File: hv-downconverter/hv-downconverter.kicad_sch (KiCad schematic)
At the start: 24 parts, among them J1 Conn_01x02_Pin, J2 Conn_01x02_Pin, Q3 Q_NMOS_GSD, Q4 Q_NMOS_GSD, U1 LM5116MHX/NOPB

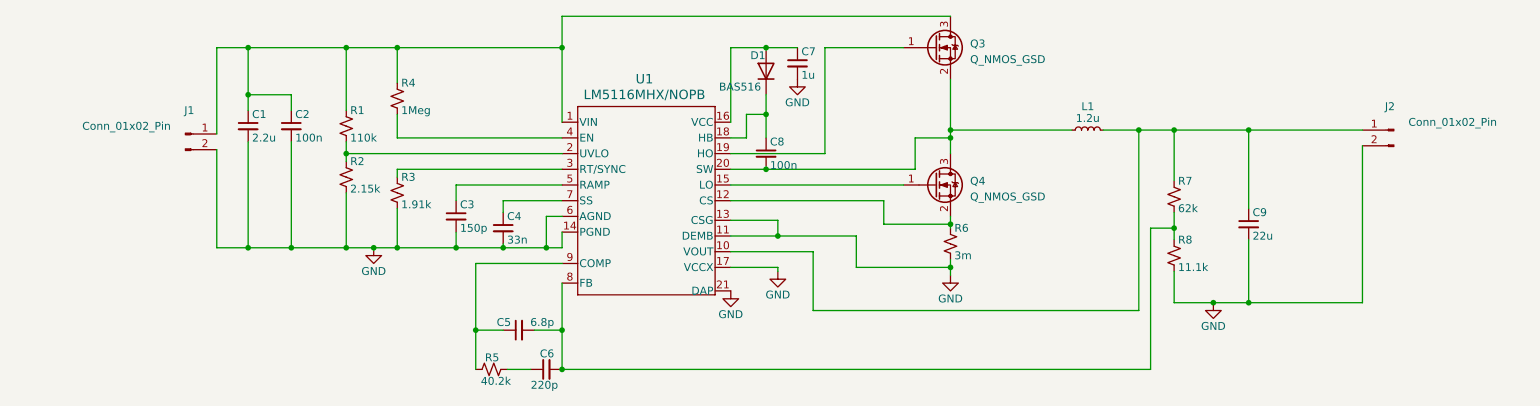
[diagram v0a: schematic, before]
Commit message: nearly at production
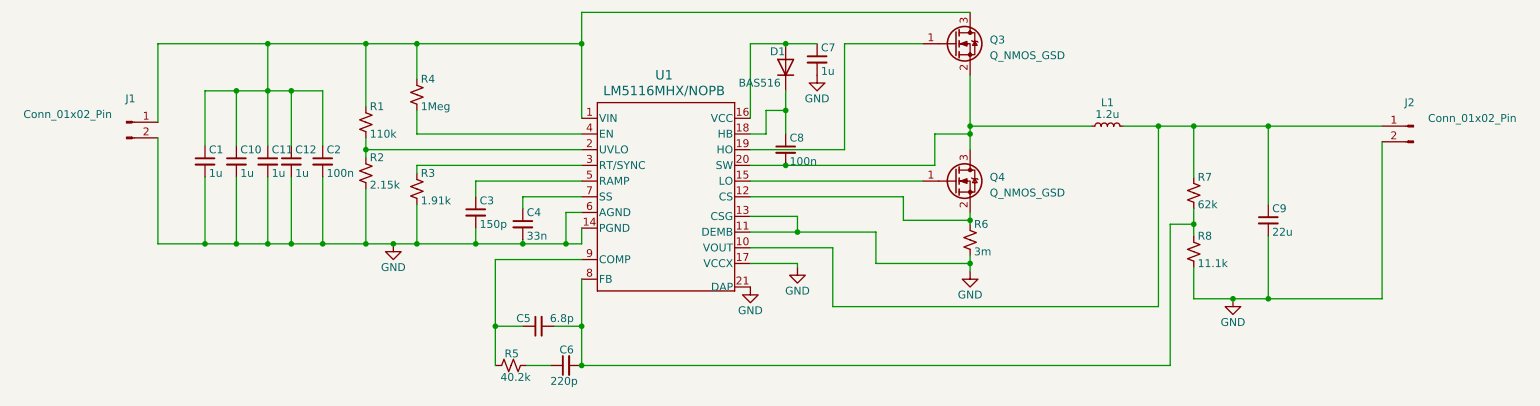
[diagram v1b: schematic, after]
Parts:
- added C10, C11, C12: 1u, Capacitor_SMD:C_2220_5750Metric, symbol Device:C_Small
- C1: value 2.2u -> 1u; footprint Capacitor_SMD:C_1210_3225Metric -> Capacitor_SMD:C_2220_5750Metric
- C2: footprint Capacitor_SMD:C_0603_1608Metric -> Capacitor_SMD:C_0805_2012Metric
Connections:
- net GND: now also C10.2, C11.2, C12.2
- net at C1.1, C2.1, J1.1 (Pin_1)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: now also C10.1, C11.1, C12.1
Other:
- moved on the sheet: C1, C2, C3, C4, C5, C6, C7, C8, C9, D1, J1, J2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
